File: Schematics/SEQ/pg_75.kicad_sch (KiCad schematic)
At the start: 16 parts, among them U7601 93S48, U7602 93S48, U7603 93S48, U7604 93S48, U7605 F244, U7606 F04, U7607 F02, U7608 F00, U7609 F02, U7610 F51, U7611 F74, U7612 F74, U7613 F74, U7614 F04, U7615 F02, U7616 F51

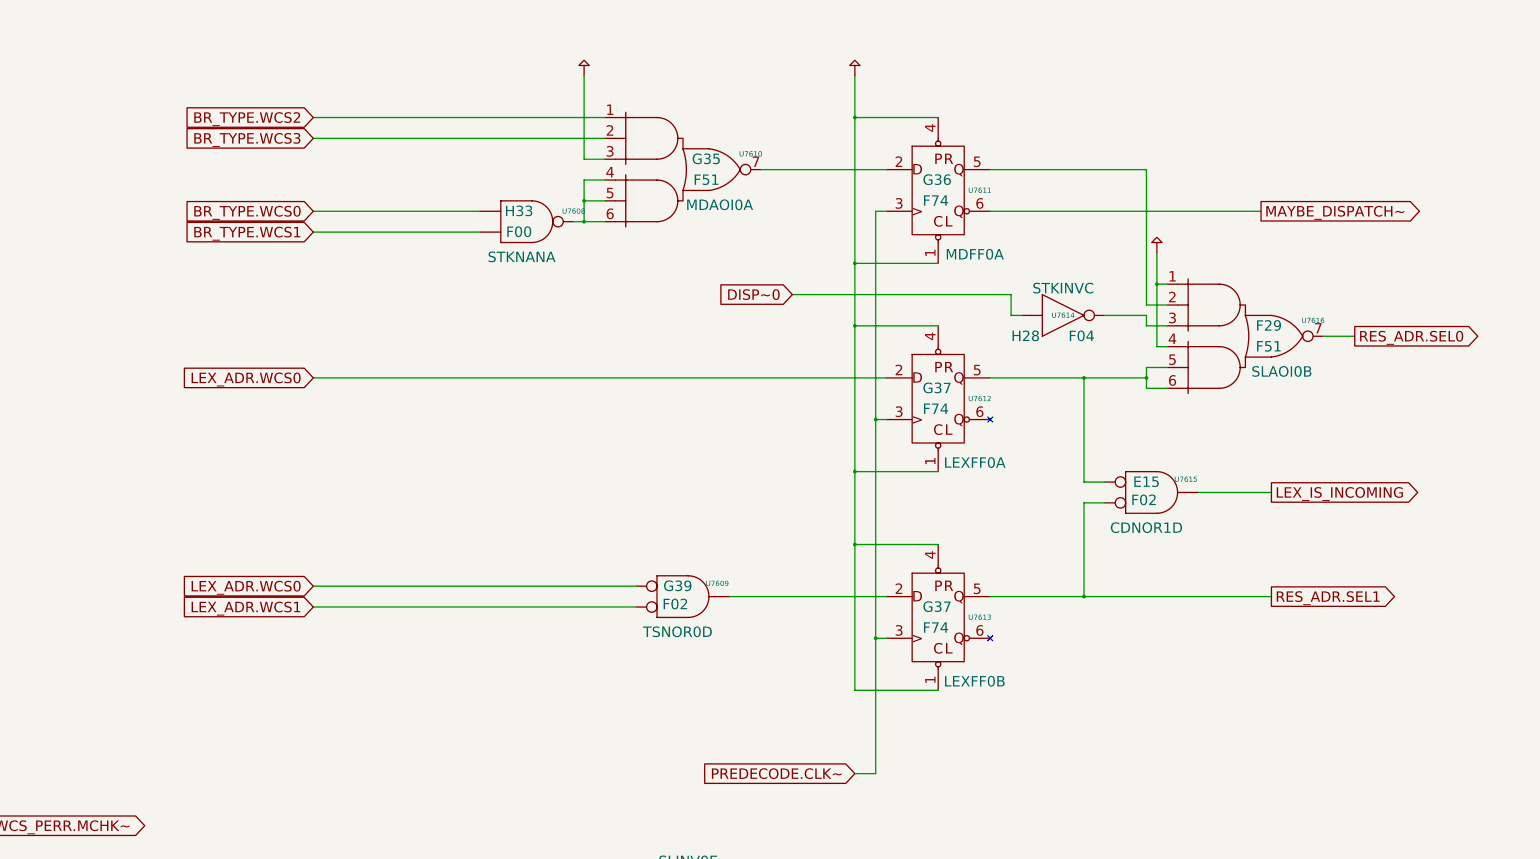
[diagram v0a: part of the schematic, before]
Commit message: Much work on SEQ
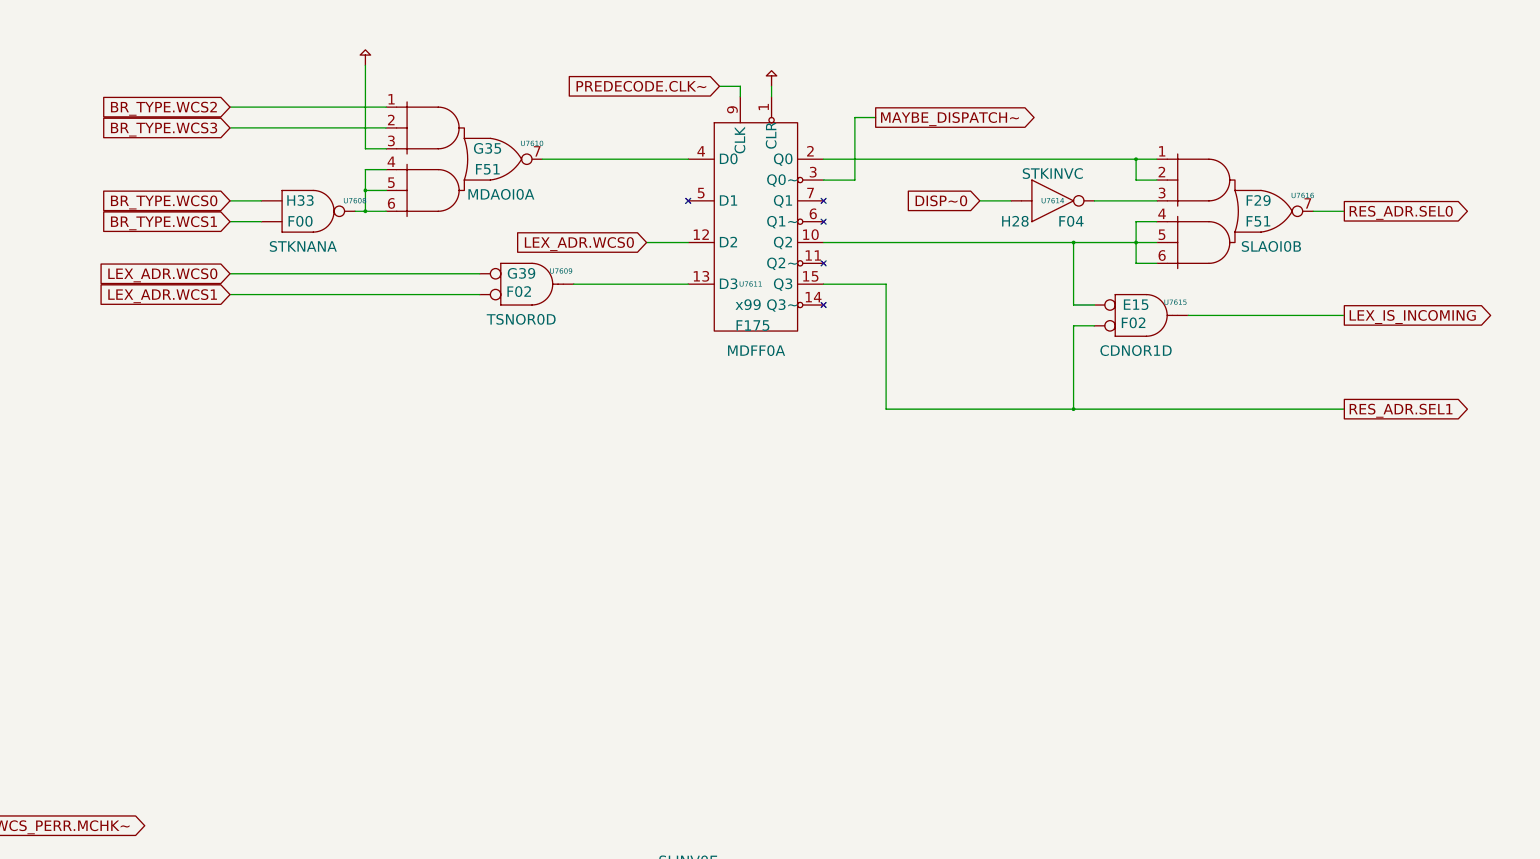
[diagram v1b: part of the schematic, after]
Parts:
- removed U7612, U7613: F74, symbol r1000:F74
- U7611: value F74 -> F175; symbol r1000:F74 -> r1000:F175; Location G36 -> x99
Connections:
- net LEX_ADR.WCS0: now also U7611.12 (D2)
- net MAYBE_DISPATCH~: now also U7611.3 (Q0~); no longer U7611.6 (Q_)
- net PREDECODE.CLK~: now also U7611.9 (CLK); no longer U7611.3 (CLK)
- net PU: no longer U7611.4 (PR_), U7616.1 (A1), U7616.4 (B1)
- net RES_ADR.SEL1: now also U7611.15 (Q3)
- net at U7609.3 (Q): now also U7611.13 (D3)
- net at U7610.7 (Q): now also U7611.4 (D0); no longer U7611.2 (D)
- net at U7616.2 (A2): now also U7611.2 (Q0), U7616.1 (A1); no longer U7611.5 (Q)
- net at U7615.1 (D0), U7616.5 (B2), U7616.6 (B3): now also U7611.10 (Q2), U7616.4 (B1)
- no-connect marks 6 -> 9
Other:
- moved on the sheet: U7608, U7609, U7610, U7614, U7615, U7616
